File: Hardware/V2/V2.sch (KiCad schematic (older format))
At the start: 61 parts, among them J1 USB_B_Mini, J2 I2C_OLED, Q1 MMBT2222, SW1 SW_Push_Dual, SW2 SW_Push_Dual, SW3 SW_Push_Dual, U1 ATmega32U4-AU, U2 LIS3DH, U3 DHT11, Y1 16Mhz

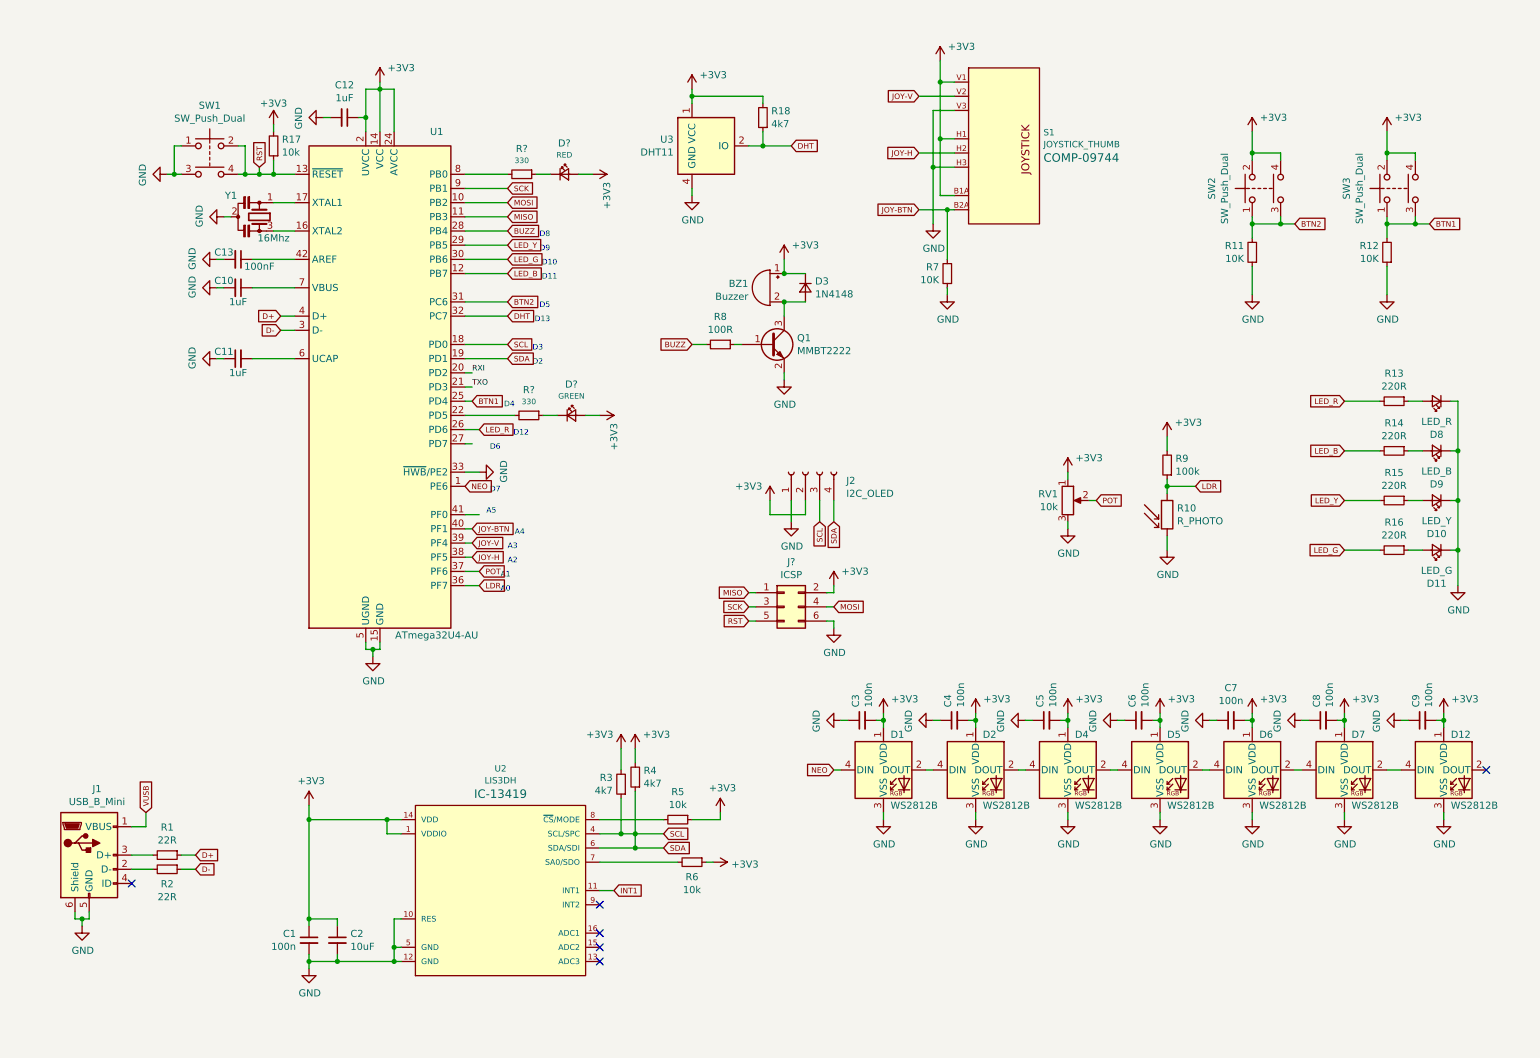
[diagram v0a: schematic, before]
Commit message: Esquema Terminado
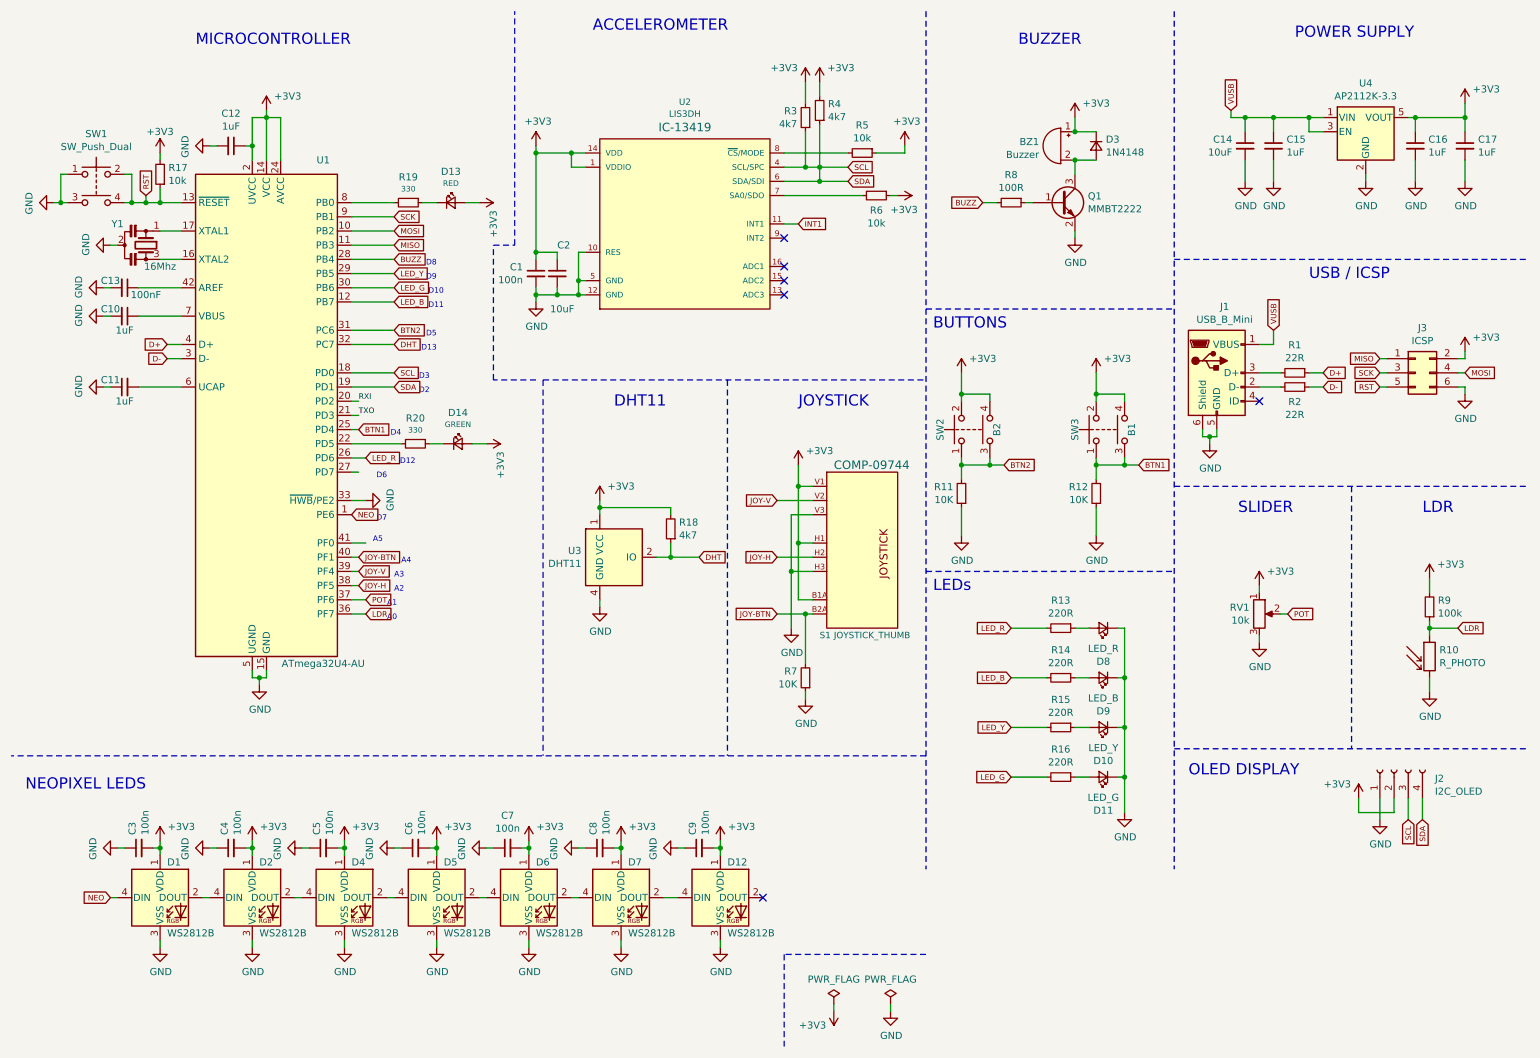
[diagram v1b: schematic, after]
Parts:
- added C14: 10uF, symbol device:C_Small
- added C15, C16, C17: 1uF, symbol device:C_Small
- added U4: AP2112K-3.3, Package_TO_SOT_SMD:SOT-23-5, symbol Regulator_Linear:AP2112K-3.3
- SW2: value SW_Push_Dual -> B2
- SW3: value SW_Push_Dual -> B1
- gave numbers to parts that had none: 5
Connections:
- net +3V3: now also C16.1, C17.1, U4.5 (VOUT)
- net GND: now also C14.2, C15.2, C16.2, C17.2, U4.2 (GND)
- net VUSB: now also C14.1, C15.1, U4.1 (VIN), U4.3 (EN)
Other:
- note added: "ACCELEROMETER"
- note added: "BUTTONS"
- note added: "BUZZER"
- note added: "DHT11"
- note added: "JOYSTICK"
- note added: "LDR"
- note added: "LEDs"
- note added: "MICROCONTROLLER"
- note added: "NEOPIXEL LEDS"
- note added: "OLED DISPLAY"
- note added: "POWER SUPPLY"
- note added: "SLIDER"
- note added: "USB / ICSP"
- moved on the sheet: BZ1, C1, C10, C11, C12, C13, C2, C3, C4, C5, C6, C7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
